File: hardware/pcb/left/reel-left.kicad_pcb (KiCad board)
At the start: 2 copper layers, 145.9 x 95.9 mm, 54 parts, among them J1 Conn_01x02, J2 Conn_01x05, SW1 SW_Push, SW10 SW_Push, SW11 SW_Push, SW12 SW_Push, SW13 SW_Push, SW14 SW_Push, SW15 SW_Push, SW16 SW_Push, SW17 SW_Push, SW18 SW_Push, SW19 SW_Push, SW2 SW_Push, SW20 SW_Push, SW21 SW_Push, SW22 SW_Push, SW24 SW_SPDT, SW25 RotaryEncoder, SW3 SW_Push, SW4 SW_Push, SW5 SW_Push, SW6 SW_Push, SW7 SW_Push, SW8 SW_Push, SW9 SW_Push

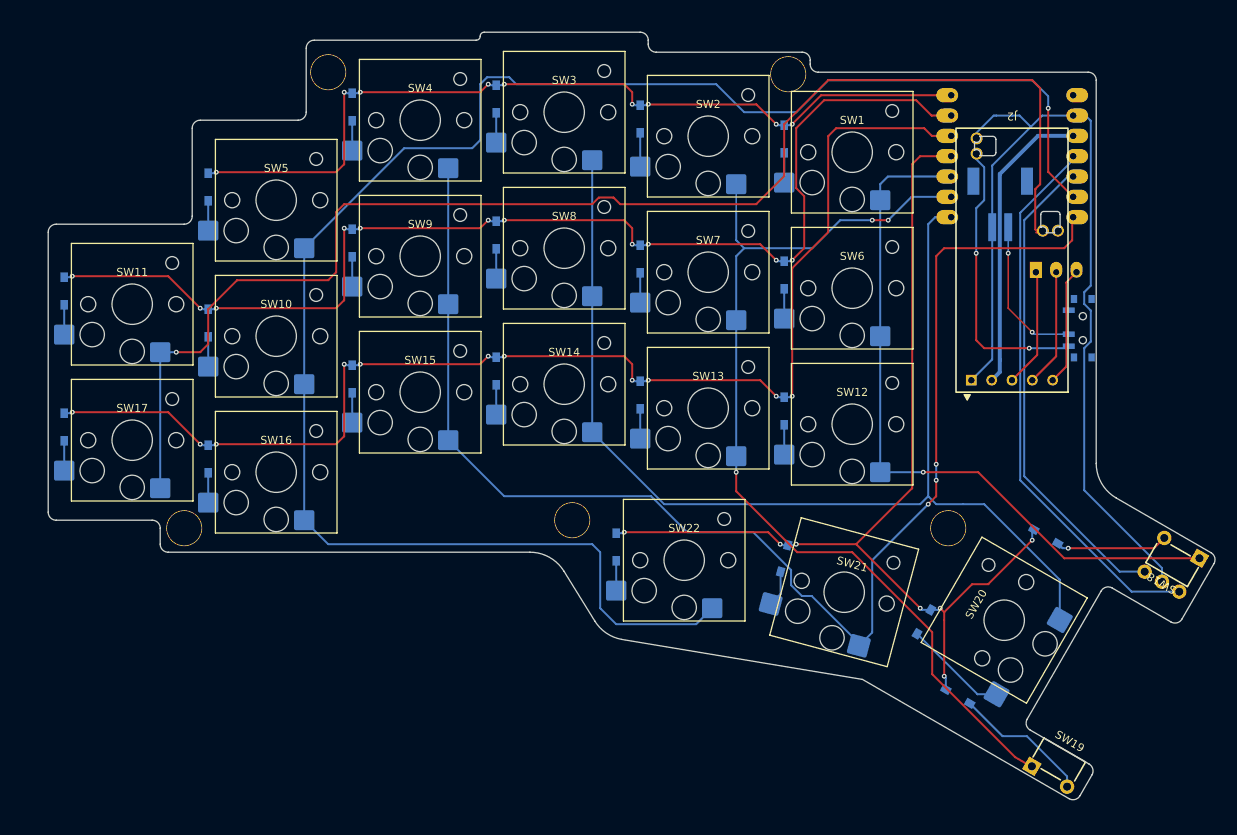
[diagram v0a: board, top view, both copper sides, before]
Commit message: Publish current hardware and fabrication assets
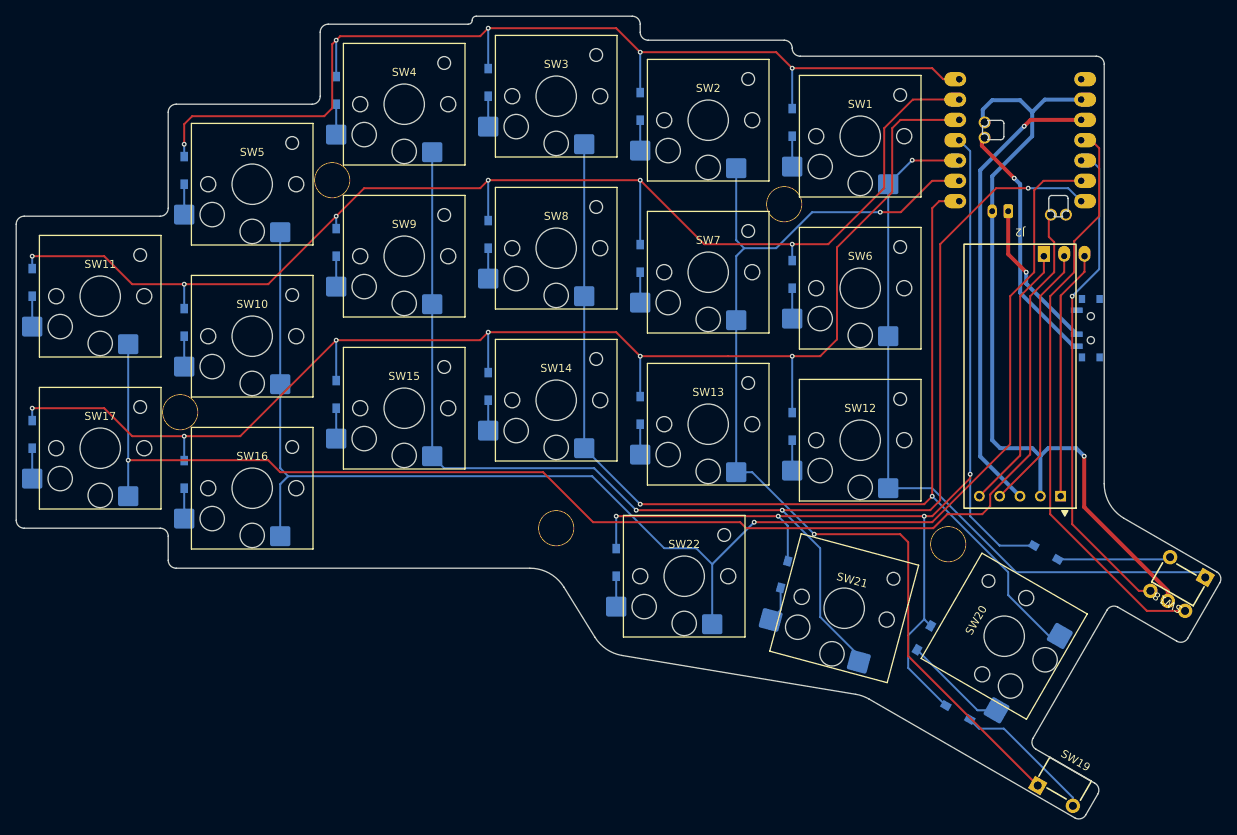
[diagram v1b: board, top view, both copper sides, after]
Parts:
- J1: footprint reel:JST_S2B-PH-SM4-TB -> Connector_JST:JST_PH_S2B-PH-K_1x02_P2.00mm_Horizontal
- moved Ref** 16.3 mm to (169.0, 74.5)
- moved J2 14.5 mm to (198.5, 111.0)
- moved Ref** 14.5 mm to (93.5, 100.5)
- moved Ref** 13.5 mm to (112.5, 71.5)
- moved D11 4.14 mm to (75.0, 81.5)
- moved SW11 4.12 mm to (83.5, 86.0)
- moved SW17 4.12 mm to (83.5, 105.0)
- moved D17 4.11 mm to (75.0, 100.5)
- moved D5 3.65 mm to (94.0, 67.5)
- moved SW16 3.61 mm to (102.5, 110.0)
- moved SW5 3.61 mm to (102.5, 72.0)
- moved D16 3.57 mm to (94.0, 105.5)
- moved D10 3.00 mm to (94.0, 86.5)
- moved SW10 3.00 mm to (102.5, 91.0)
- moved D4 2.88 mm to (113.0, 57.5)
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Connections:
- J2 pad 1: GND -> SI
- J2 pad 2: 3.3V -> SCK
- J2 pad 3: SI -> 3.3V
- J2 pad 4: SCK -> GND
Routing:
- net Col4: track 219.4 -> 186.7 mm
- net Row0: track 107.6 -> 132.9 mm, vias 9 -> 5
- net 3.3V: track 37.3 -> 58.0 mm, vias 0 -> 1
- net SCK: track 14.7 -> 33.3 mm
- net SI: track 14.9 -> 33.3 mm
- net Row2: track 156.9 -> 174.4 mm, vias 11 -> 6
- net CS: track 14.7 -> 31.2 mm
- net GND: track 114.3 -> 98.8 mm, vias 0 -> 1
- net Row3: track 127.2 -> 141.6 mm, vias 7 -> 4
- net Row1: track 146.3 -> 159.2 mm, vias 11 -> 6
- net Col3: track 170.7 -> 180.9 mm
- net Col1: track 121.9 -> 131.4 mm, vias 3 -> 2
- net Col2: track 143.2 -> 149.4 mm, vias 0 -> 2
- net VBAT_SW: track 36.1 -> 30.9 mm, vias 2 -> 1
- net RotB: track 69.1 -> 72.8 mm
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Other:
- board size 145.9 x 95.9 mm -> 150.6 x 100.3 mm
